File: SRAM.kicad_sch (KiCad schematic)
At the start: 11 parts, among them U31 CY7C199, U310 CY7C199, U311 CY7C199, U312 CY7C199, U313 74LS138, U32 CY7C199, U33 CY7C199, U34 CY7C199, U35 74LS138, U36 74LS138, U39 CY7C199

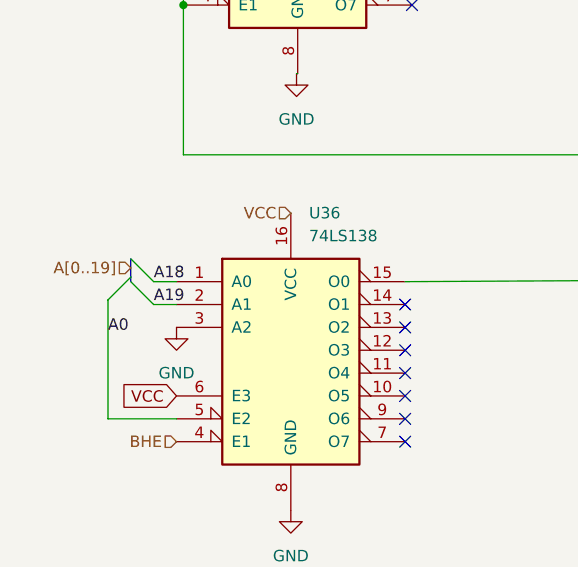
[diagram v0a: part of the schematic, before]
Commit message: Added bullet 6
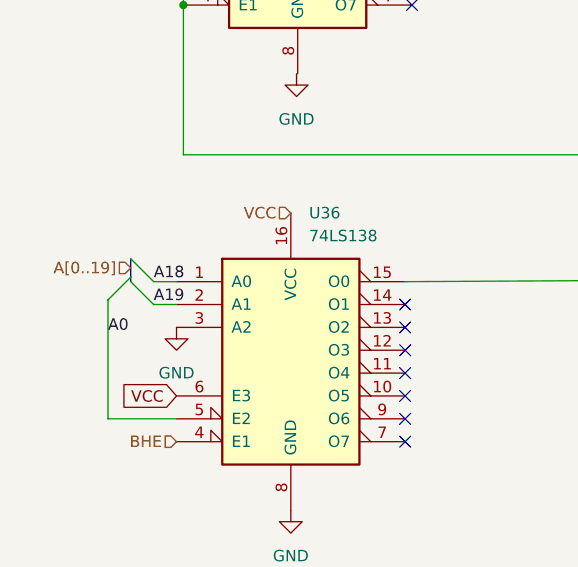
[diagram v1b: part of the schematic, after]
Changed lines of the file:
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@@
     (effects (font (size 1.27 1.27)) (justify left bottom))
   )
-  (label "A18" (at 25.1523 152.146 0)
+  (label "A18" (at 25.146 152.146 0)
     (effects (font (size 1.27 1.27)) (justify left bottom))
   )
@@
     (effects (font (size 1.27 1.27)) (justify left bottom))
   )
-  (label "A19" (at 25.1523 154.686 0)
-    (effects (font (size 1.27 1.27)) (justify left bottom))
-  )
+  (label "A19" (at 25.146 154.686 0)
+    (effects (font (size 1.27 1.27)) (justify left bottom))
+  )

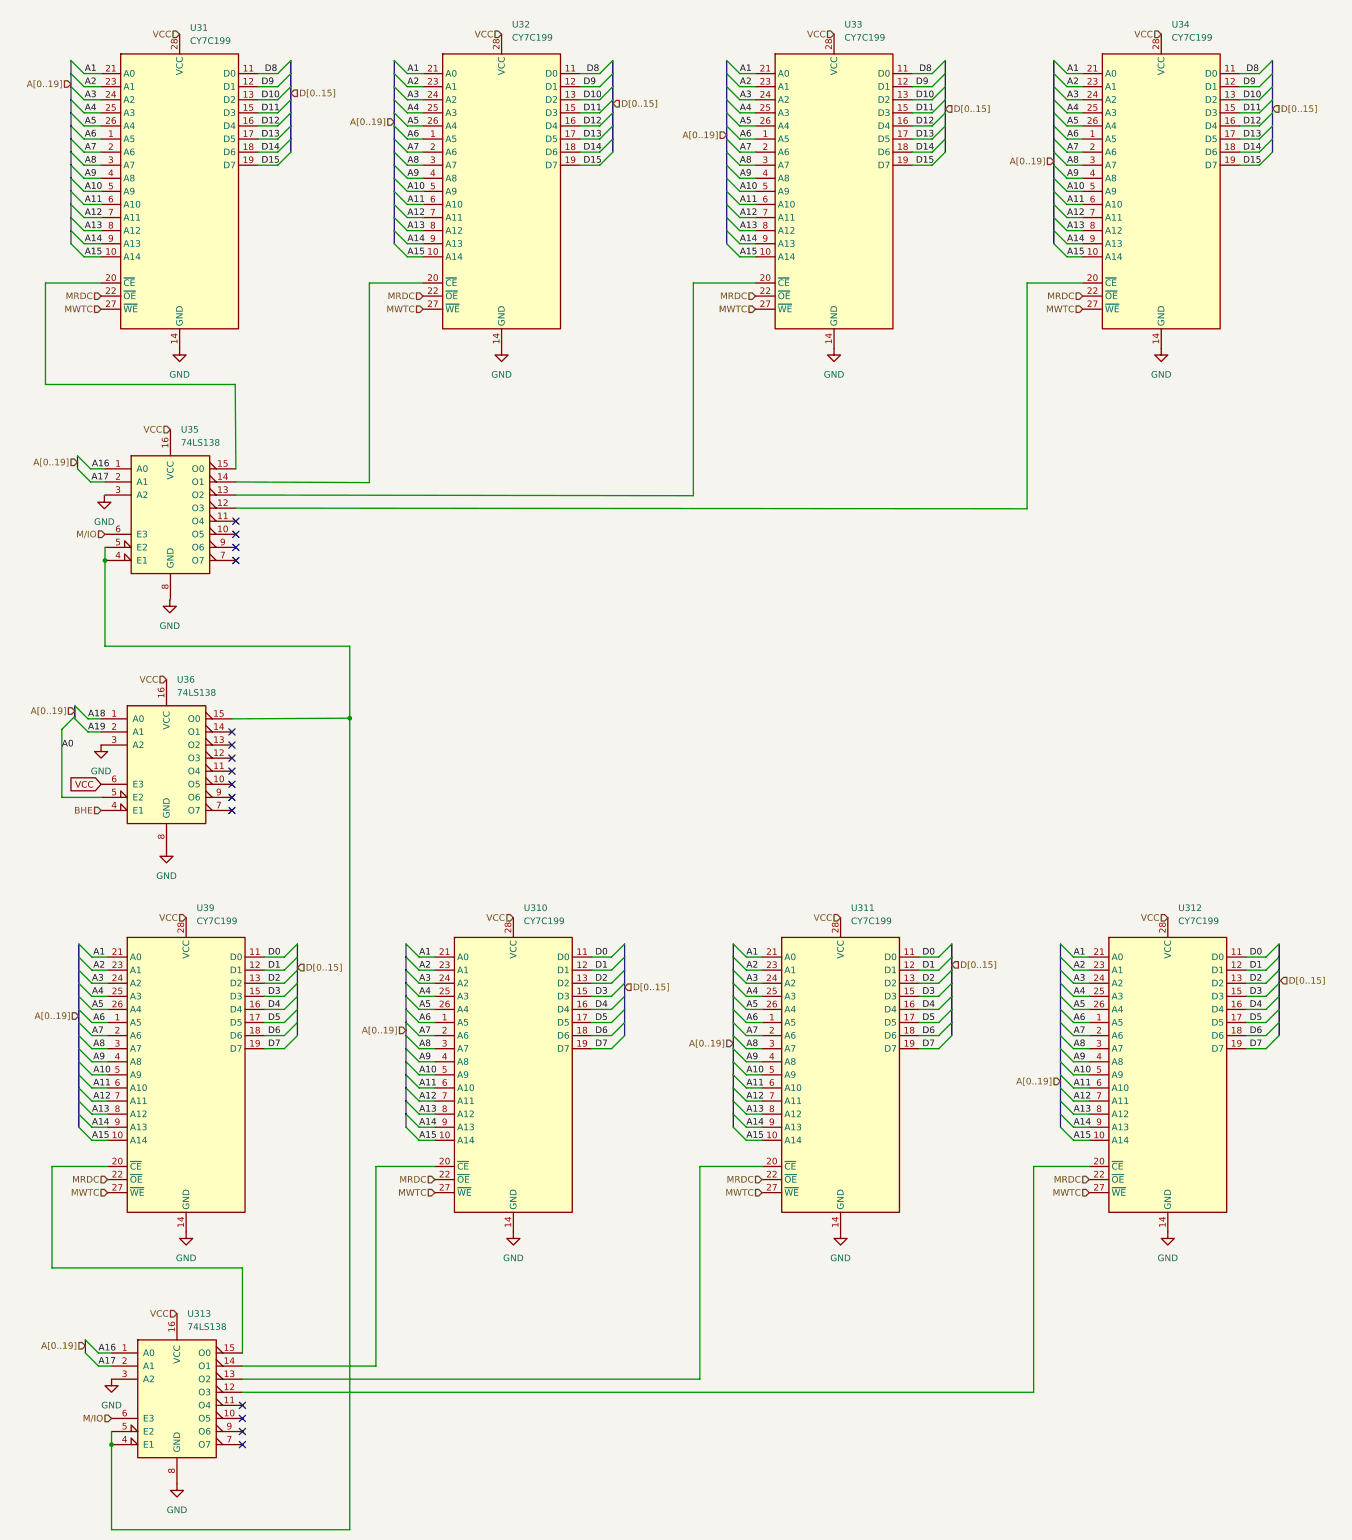
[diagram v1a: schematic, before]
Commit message: stuff
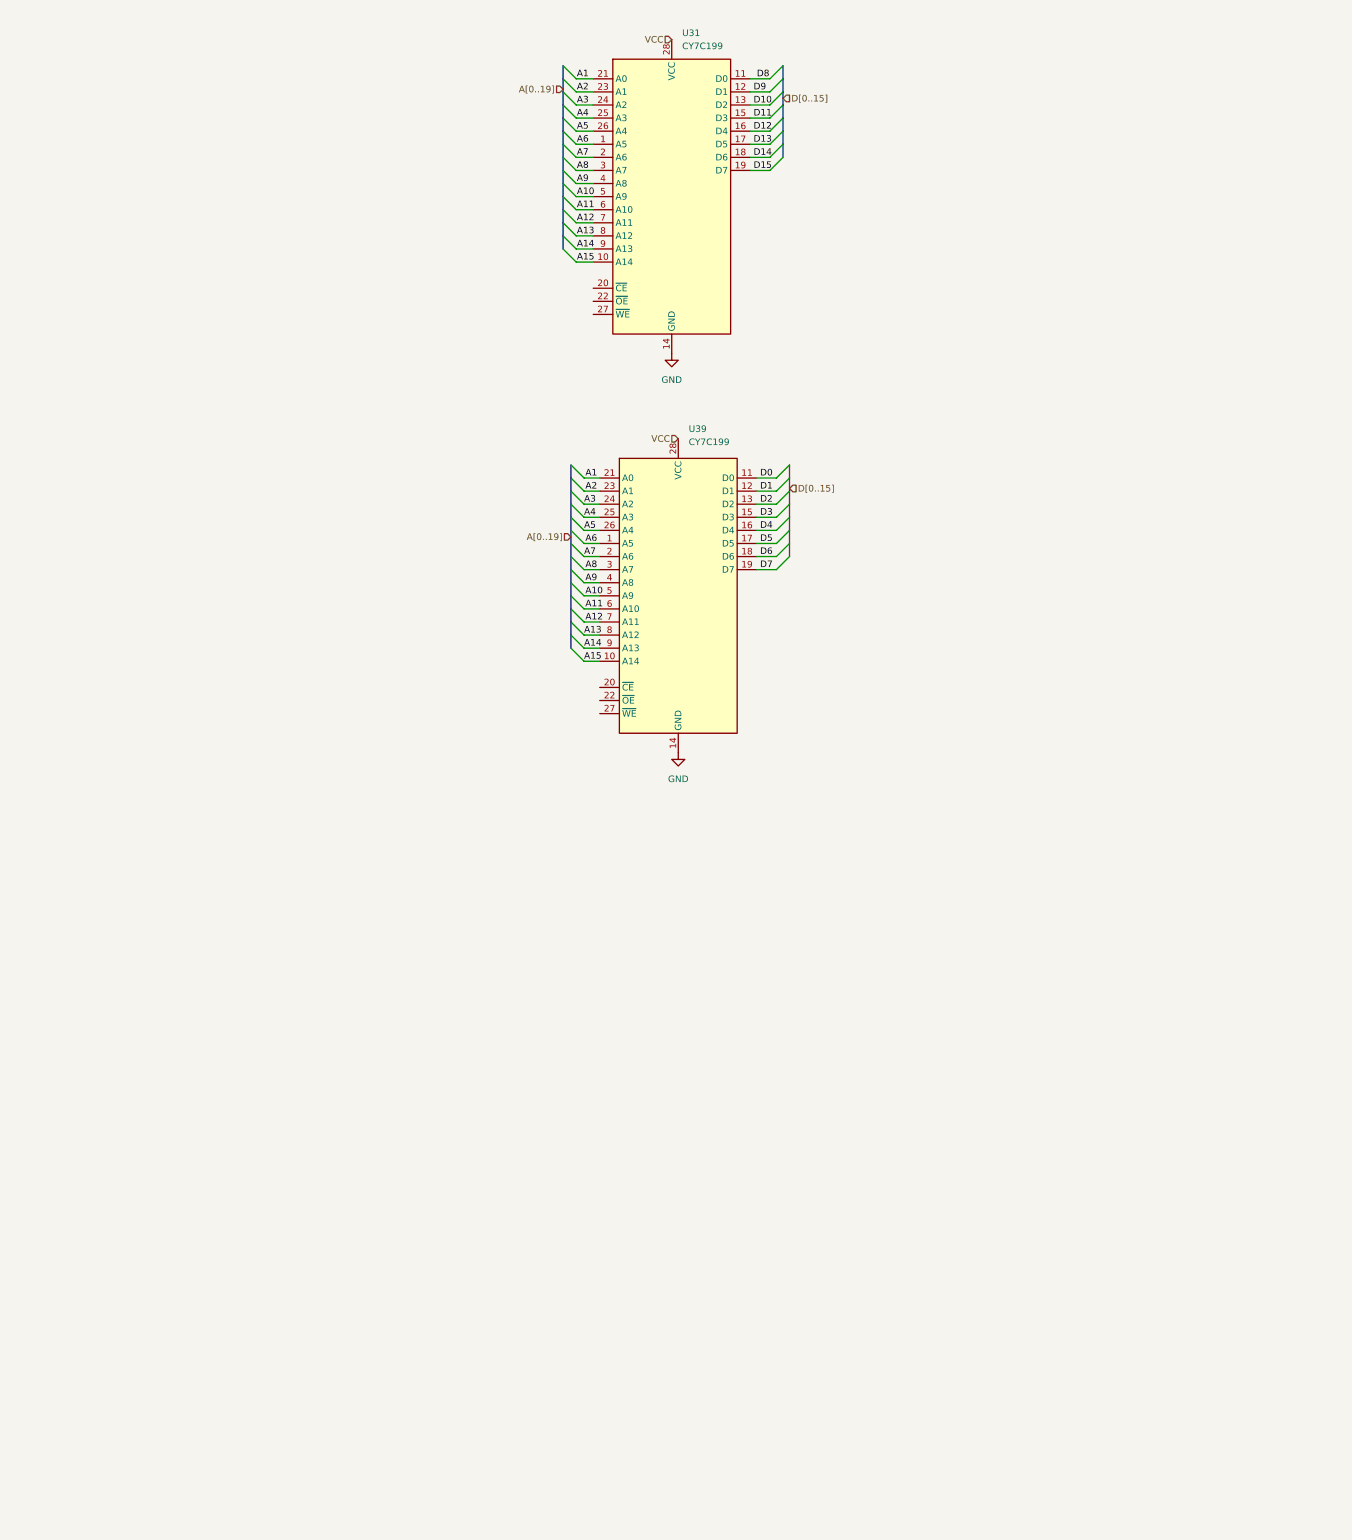
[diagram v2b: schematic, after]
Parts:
- removed U310, U311, U312, U32, U33, U34: CY7C199, symbol Memory_RAM:CY7C199
- removed U313, U35, U36: 74LS138, symbol 74xx:74LS138
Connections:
- net MRDC: no longer names the net of U31.22 (~{OE})
- net MRDC: no longer U39.22 (~{OE})
- net MWTC: no longer names the net of U31.27 (~{WE})
- net MWTC: no longer U39.27 (~{WE})
- no-connect marks 15 -> 0
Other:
- moved on the sheet: U31, U39

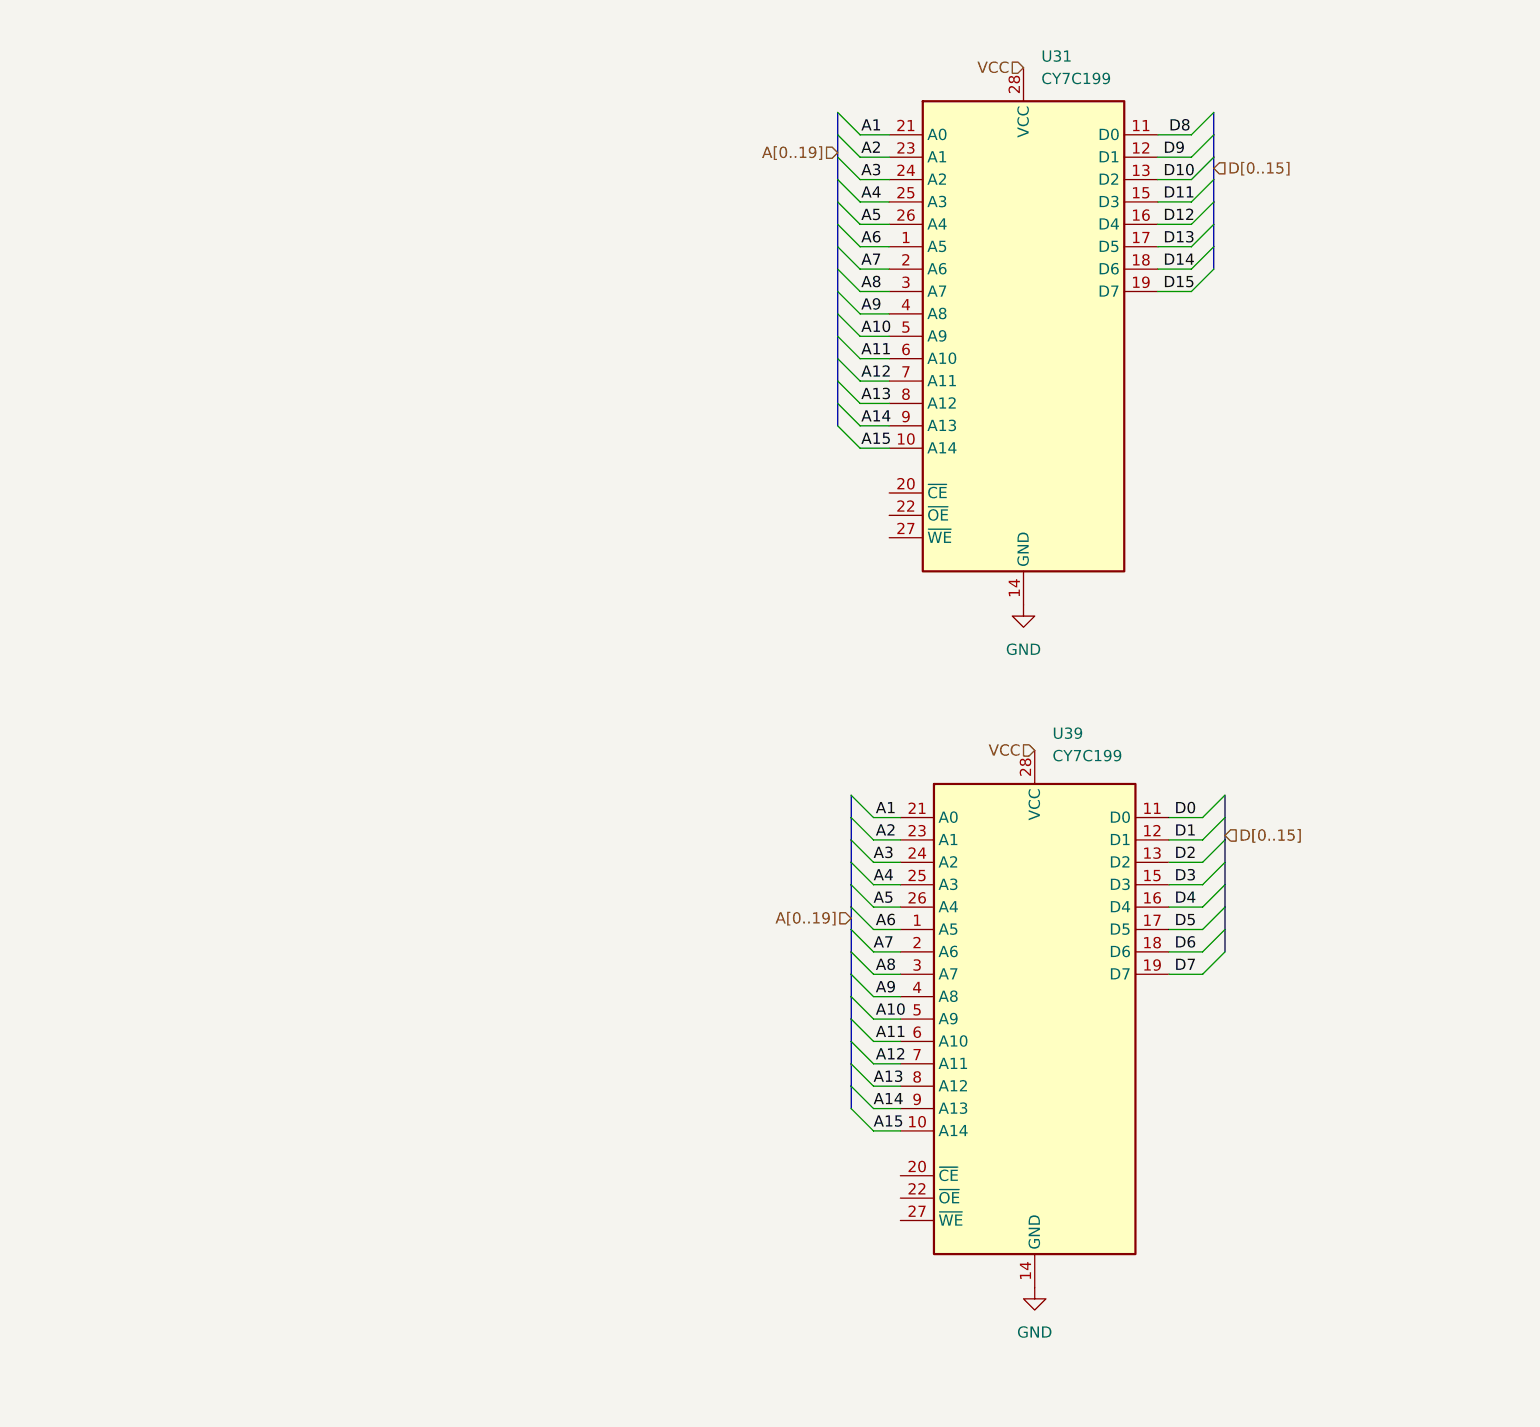
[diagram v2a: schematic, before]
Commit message: finished design
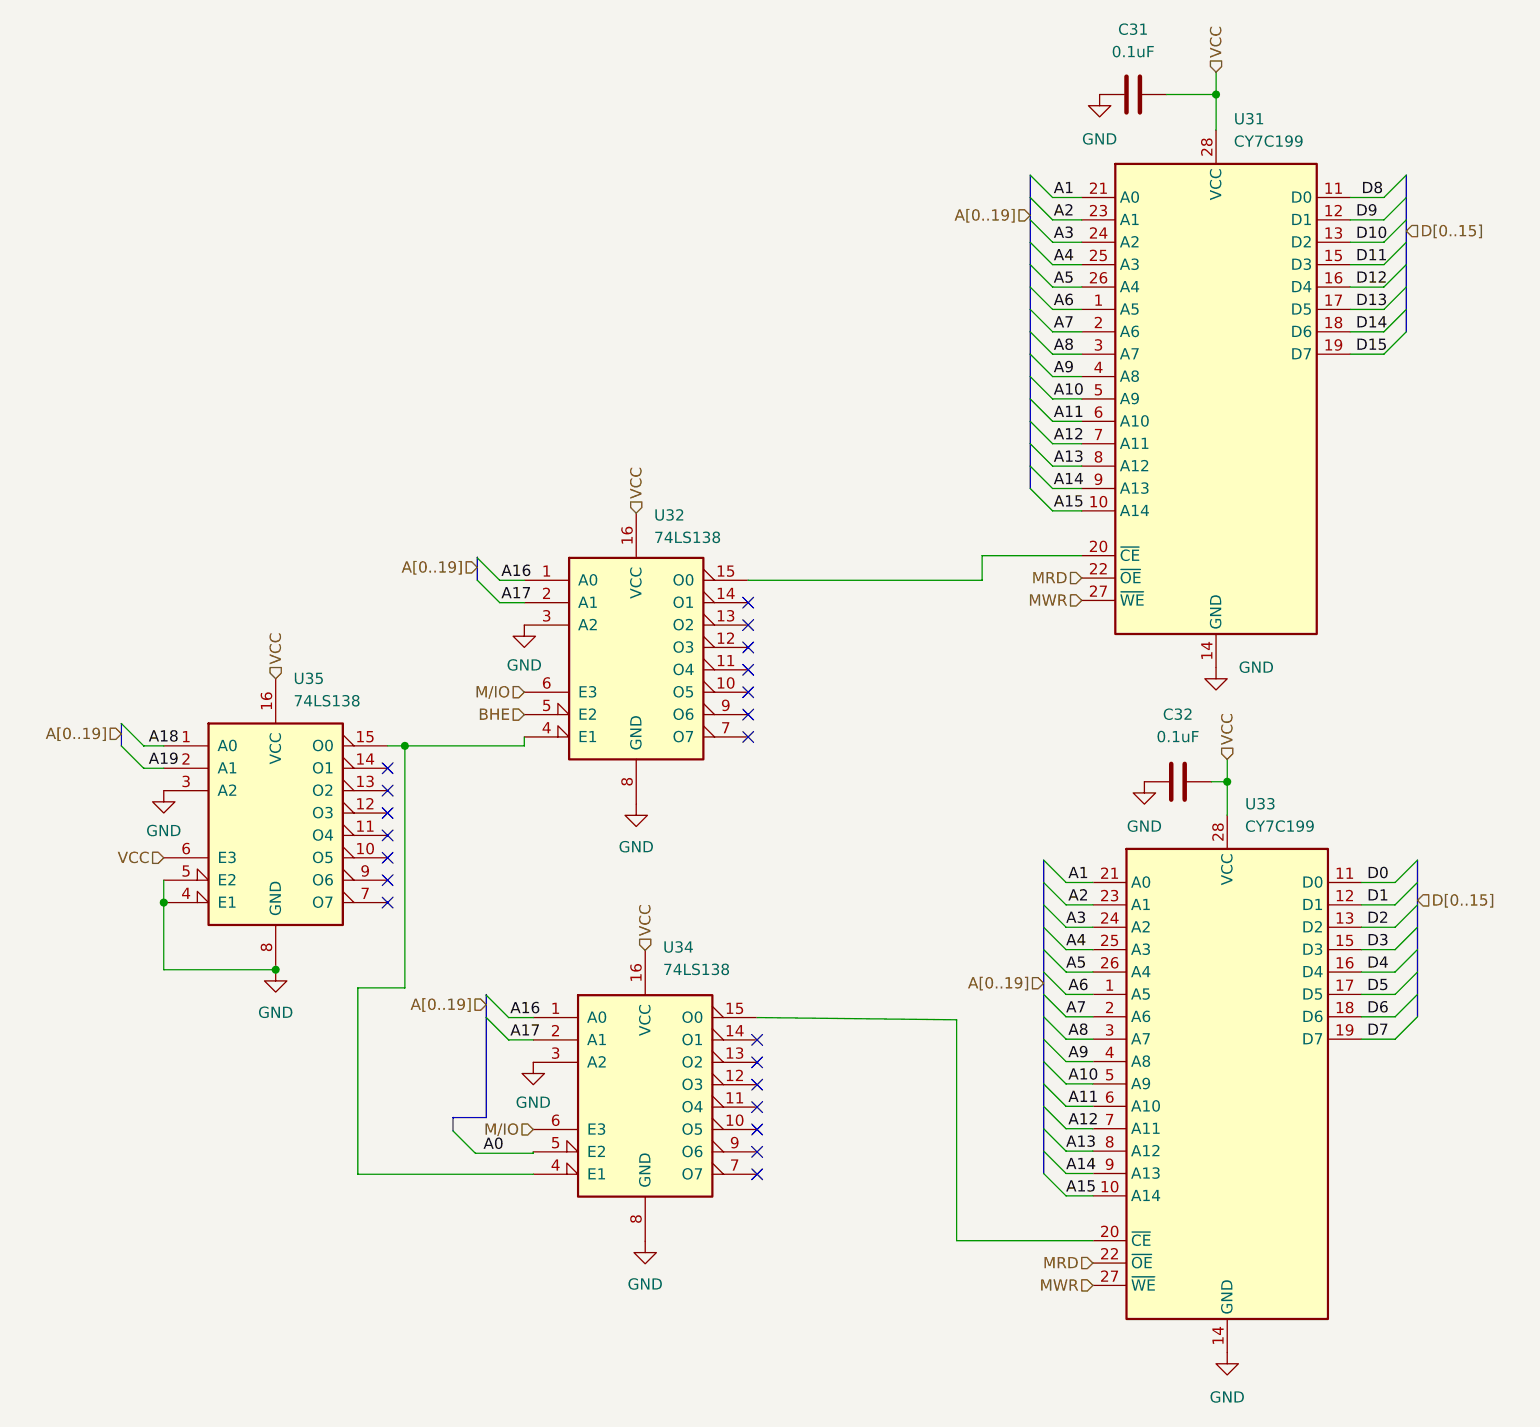
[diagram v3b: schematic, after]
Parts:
- added C31, C32: 0.1uF, Capacitor_THT:C_Axial_L3.8mm_D2.6mm_P7.50mm_Horizontal, symbol Device:C
- added U32, U34, U35: 74LS138, Package_DIP:DIP-16_W7.62mm, symbol 74xx:74LS138
- U31: footprint (none) -> Package_DIP:DIP-28_W7.62mm
- U33: renamed from U39; footprint (none) -> Package_DIP:DIP-28_W7.62mm
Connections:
- net GND: now also C31.1, C32.1, U32.3 (A2), U32.8 (GND), U34.3 (A2), U34.8 (GND), U35.3 (A2), U35.4 (E1), U35.5 (E2), U35.8 (GND)
- net VCC: now also C31.2, C32.2, U32.16 (VCC), U34.16 (VCC), U35.16 (VCC), U35.6 (E3)
- net at U31.20 (~{CE}): now also U32.15 (O0)
- net MRD: now reaches U31.22 (~{OE})
- net MRD: now also U33.22 (~{OE})
- net MWR: now reaches U31.27 (~{WE})
- net MWR: now also U33.27 (~{WE})
- net at U33.20 (~{CE}): now also U34.15 (O0)
- new net: U32.4 (E1), U34.4 (E1), U35.15 (O0)
- new net A0: U34.5 (E2)
- new net A16: U32.1 (A0), U34.1 (A0)
- new net A17: U32.2 (A1), U34.2 (A1)
- new net A18: U35.1 (A0)
- new net A19: U35.2 (A1)
- new net BHE: U32.5 (E2)
- new net M/IO: U32.6 (E3), U34.6 (E3)
- no-connect marks 0 -> 21
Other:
- moved on the sheet: U31, U33
